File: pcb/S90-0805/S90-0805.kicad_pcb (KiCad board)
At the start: 2 copper layers, 100 x 40 mm, 9 parts

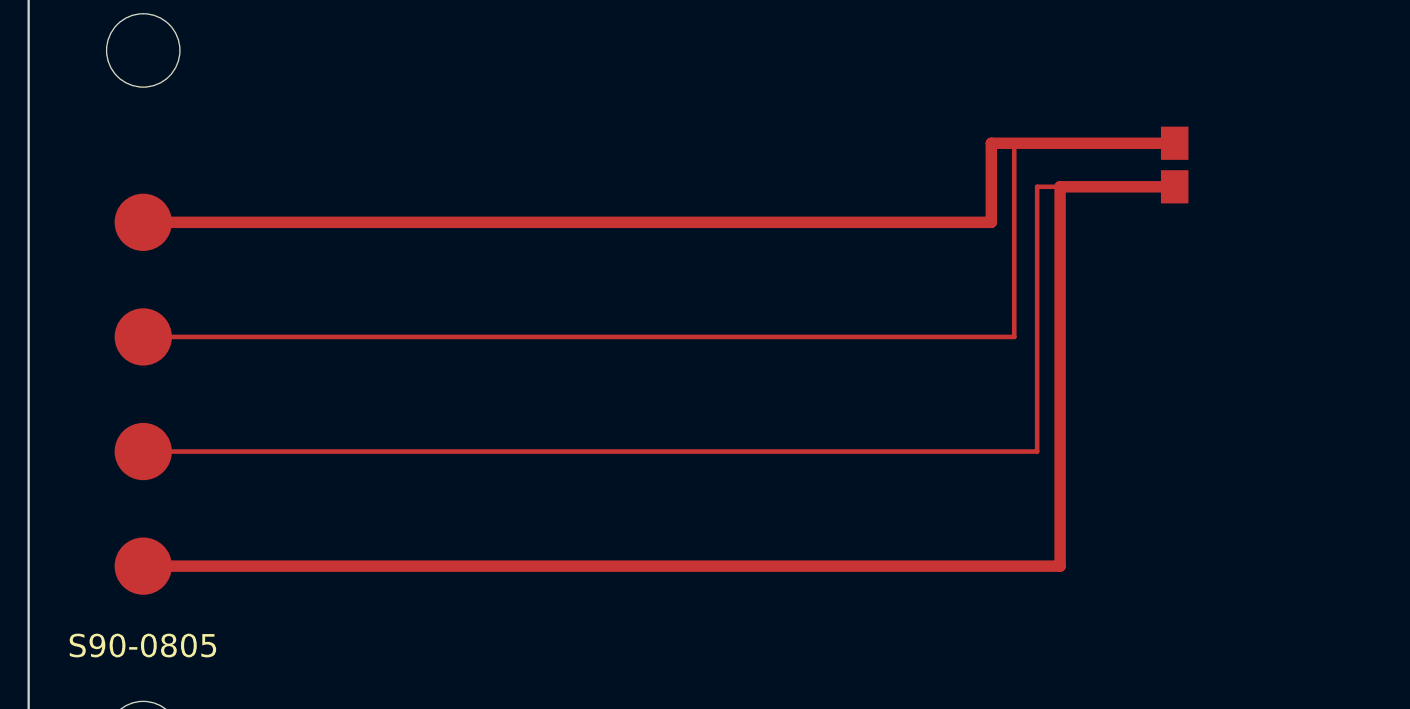
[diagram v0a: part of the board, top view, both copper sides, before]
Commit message: v0.3.1 — PCB CAD & JLCPCB Fabrication Package
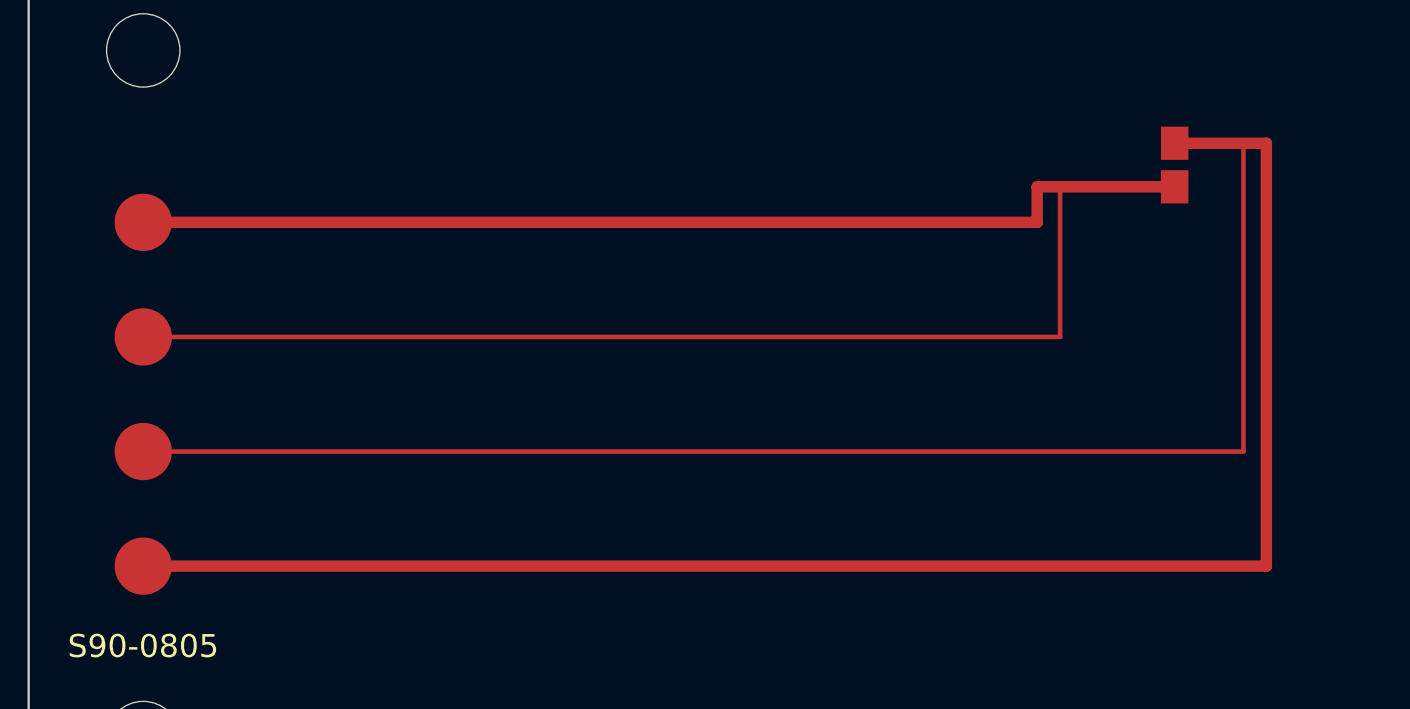
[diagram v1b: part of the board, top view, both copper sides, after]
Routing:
- net DRIVE_SENSE_MINUS: track 118.1 -> 135.9 mm
- net DRIVE_SENSE_PLUS: track 101.9 -> 98.1 mm
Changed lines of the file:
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@@
 		(pad "1" smd rect (at -0.95 0) (size 1.2 1.45) (layers "F.Cu" "F.Paste" "F.Mask") (net 1 "DRIVE_SENSE_PLUS"))
 		(pad "2" smd rect (at 0.95 0) (size 1.2 1.45) (layers "F.Cu" "F.Paste" "F.Mask") (net 2 "DRIVE_SENSE_MINUS"))
+		(model "/Applications/KiCad/KiCad.app/Contents/SharedSupport/3dmodels/Capacitor_SMD.3dshapes/C_0805_2012Metric.step"
+			(offset (xyz 0 0 0))
+			(scale (xyz 1 1 1))
+			(rotate (xyz 0 0 0))
+		)
 	)
 	(footprint "SC4:EdgeContact_2.5mm_Round" (layer "F.Cu")
@@
 		(pad "1" smd circle (at 0 0) (size 2.5 2.5) (layers "F.Cu" "F.Mask") (net 2 "DRIVE_SENSE_MINUS"))
 	)
-	(segment (start 5.0 12.5) (end 42.0 12.5) (width 0.5) (layer "F.Cu") (net 1))
-	(segment (start 42.0 12.5) (end 42.0 9.05) (width 0.5) (layer "F.Cu") (net 1))
-	(segment (start 42.0 9.05) (end 50.0 9.05) (width 0.5) (layer "F.Cu") (net 1))
-	(segment (start 5.0 17.5) (end 43.0 17.5) (width 0.2) (layer "F.Cu") (net 1))
-	(segment (start 43.0 17.5) (end 43.0 9.05) (width 0.2) (layer "F.Cu") (net 1))
-	(segment (start 43.0 9.05) (end 50.0 9.05) (width 0.2) (layer "F.Cu") (net 1))
-	(segment (start 5.0 22.5) (end 44.0 22.5) (width 0.2) (layer "F.Cu") (net 2))
-	(segment (start 44.0 22.5) (end 44.0 10.95) (width 0.2) (layer "F.Cu") (net 2))
-	(segment (start 44.0 10.95) (end 50.0 10.95) (width 0.2) (layer "F.Cu") (net 2))
-	(segment (start 5.0 27.5) (end 45.0 27.5) (width 0.5) (layer "F.Cu") (net 2))
-	(segment (start 45.0 27.5) (end 45.0 10.95) (width 0.5) (layer "F.Cu") (net 2))
-	(segment (start 45.0 10.95) (end 50.0 10.95) (width 0.5) (layer "F.Cu") (net 2))
+	(segment (start 5.0 12.5) (end 44.0 12.5) (width 0.5) (layer "F.Cu") (net 1))
+	(segment (start 44.0 12.5) (end 44.0 10.95) (width 0.5) (layer "F.Cu") (net 1))
+	(segment (start 44.0 10.95) (end 50.0 10.95) (width 0.5) (layer "F.Cu") (net 1))
+	(segment (start 5.0 17.5) (end 45.0 17.5) (width 0.2) (layer "F.Cu") (net 1))
+	(segment (start 45.0 17.5) (end 45.0 10.95) (width 0.2) (layer "F.Cu") (net 1))
+	(segment (start 45.0 10.95) (end 50.0 10.95) (width 0.2) (layer "F.Cu") (net 1))
+	(segment (start 5.0 22.5) (end 53.0 22.5) (width 0.2) (layer "F.Cu") (net 2))
+	(segment (start 53.0 22.5) (end 53.0 9.05) (width 0.2) (layer "F.Cu") (net 2))
+	(segment (start 53.0 9.05) (end 50.0 9.05) (width 0.2) (layer "F.Cu") (net 2))
+	(segment (start 5.0 27.5) (end 54.0 27.5) (width 0.5) (layer "F.Cu") (net 2))
+	(segment (start 54.0 27.5) (end 54.0 9.05) (width 0.5) (layer "F.Cu") (net 2))
+	(segment (start 54.0 9.05) (end 50.0 9.05) (width 0.5) (layer "F.Cu") (net 2))
 	(gr_text "S90-0805" (at 5.0 31.0 0) (layer "F.SilkS")
 		(effects (font (size 1 1) (thickness 0.15)))
